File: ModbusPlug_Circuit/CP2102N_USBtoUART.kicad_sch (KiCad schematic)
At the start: 0 parts

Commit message: Updated USB/PD and TTL circuit
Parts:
- added C3: 4.7uF|16V, Capacitor_SMD:C_0402_1005Metric, symbol Device:C
- added C4: 100nF|16V, Capacitor_SMD:C_0402_1005Metric, symbol Device:C
- added D1, D2, D3: RED LED, LED_SMD:LED_0402_1005Metric, symbol Device:LED
- added R2: 1k 5%, Resistor_SMD:R_0402_1005Metric, symbol Device:R
- added R3: 22.1k 5%, Resistor_SMD:R_0402_1005Metric, symbol Device:R
- added R4: 47k 5%, Resistor_SMD:R_0402_1005Metric, symbol Device:R
- added RN1: 1k 5%, Resistor_SMD:R_Array_Convex_4x0402, symbol Device:R_Network04_Split
- added U2: CP2102N-Axx-xQFN20, Package_DFN_QFN:SiliconLabs_QFN-20-1EP_3x3mm_P0.5mm_EP1.8x1.8mm, symbol Interface_USB:CP2102N-Axx-xQFN20
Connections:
- new net: D2.2 (A), RN1.1 (R1)
- new net: R3.2, R4.1, U2.8 (VBUS)
- new net: D3.2 (A), RN1.1 (R1)
- new net: D1.2 (A), RN1.1 (R1)
- new net: R2.2, U2.9 (~{RST})
- new net Din_+: U2.5 (D-)
- new net Din_-: U2.4 (D+)
- new net GND: C3.2, C4.2, D1.1 (K), R4.2, U2.12 (GND), U2.21 (GND), U2.3 (GND)
- new net RS485_DE: U2.1 (RS485/GPIO.1)
- new net RXT: D3.1 (K), U2.19 (~{RXT}/GPIO.3)
- new net TXT: D2.1 (K), U2.20 (~{TXT}/GPIO.2)
- new net UART_RX: U2.17 (RXD)
- new net UART_TX: U2.18 (TXD)
- new net VBUS_in: R3.1
- new net Vin: C3.1, C4.1, R2.1, RN1.2 (R1.2), RN1.3 (R2.2), RN1.4 (R3.2), U2.6 (VDD), U2.7 (VREGIN)
- no-connect marks 0 -> 8

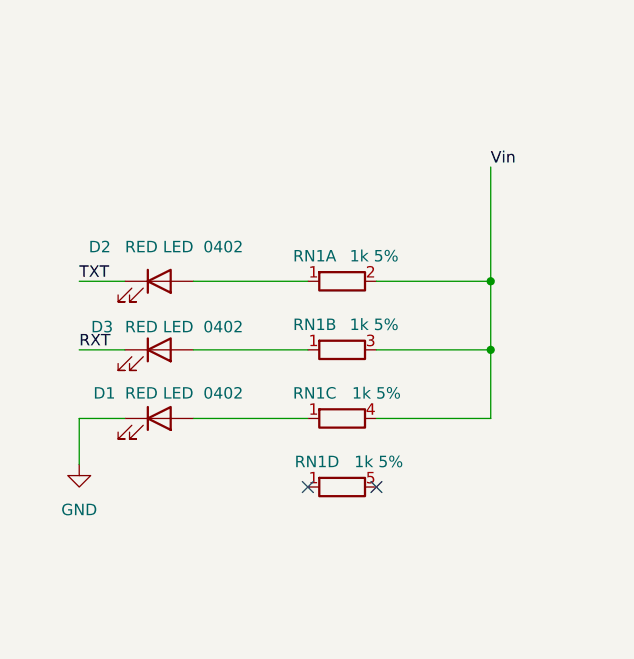
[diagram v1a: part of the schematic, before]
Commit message: pushing V0.1
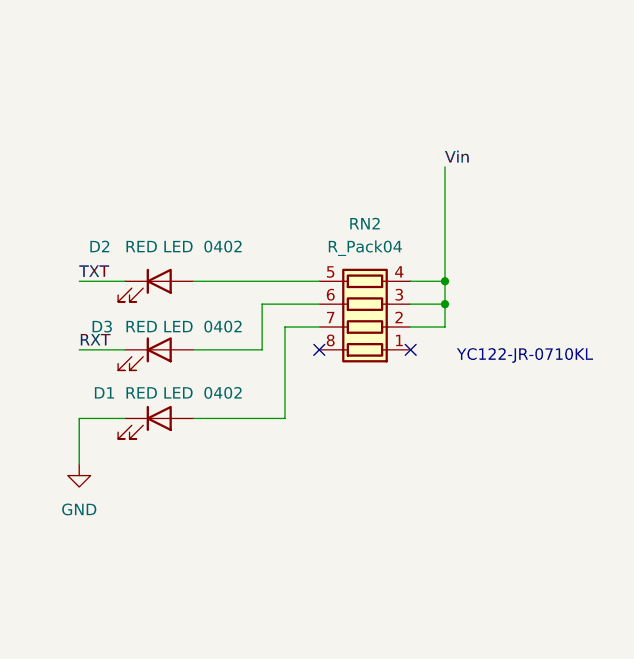
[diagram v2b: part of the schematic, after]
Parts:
- removed RN1: 1k 5%, Resistor_SMD:R_Array_Convex_4x0402, symbol Device:R_Network04_Split
- added RN2: R_Pack04, Resistor_SMD:R_Array_Convex_4x0402, symbol Device:R_Pack04
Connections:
- net Vin: now also RN2.2 (R2.1), RN2.3 (R3.1), RN2.4 (R4.1)
- net at D2.2 (A): now also RN2.5 (R4.2)
- net at D3.2 (A): now also RN2.6 (R3.2)
- net at D1.2 (A): now also RN2.7 (R2.2)
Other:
- note added: "YC122-JR-0710KL"
